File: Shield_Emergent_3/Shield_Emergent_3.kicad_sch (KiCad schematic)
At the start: 23 parts, among them J1 Conn_02x06_Counter_Clockwise

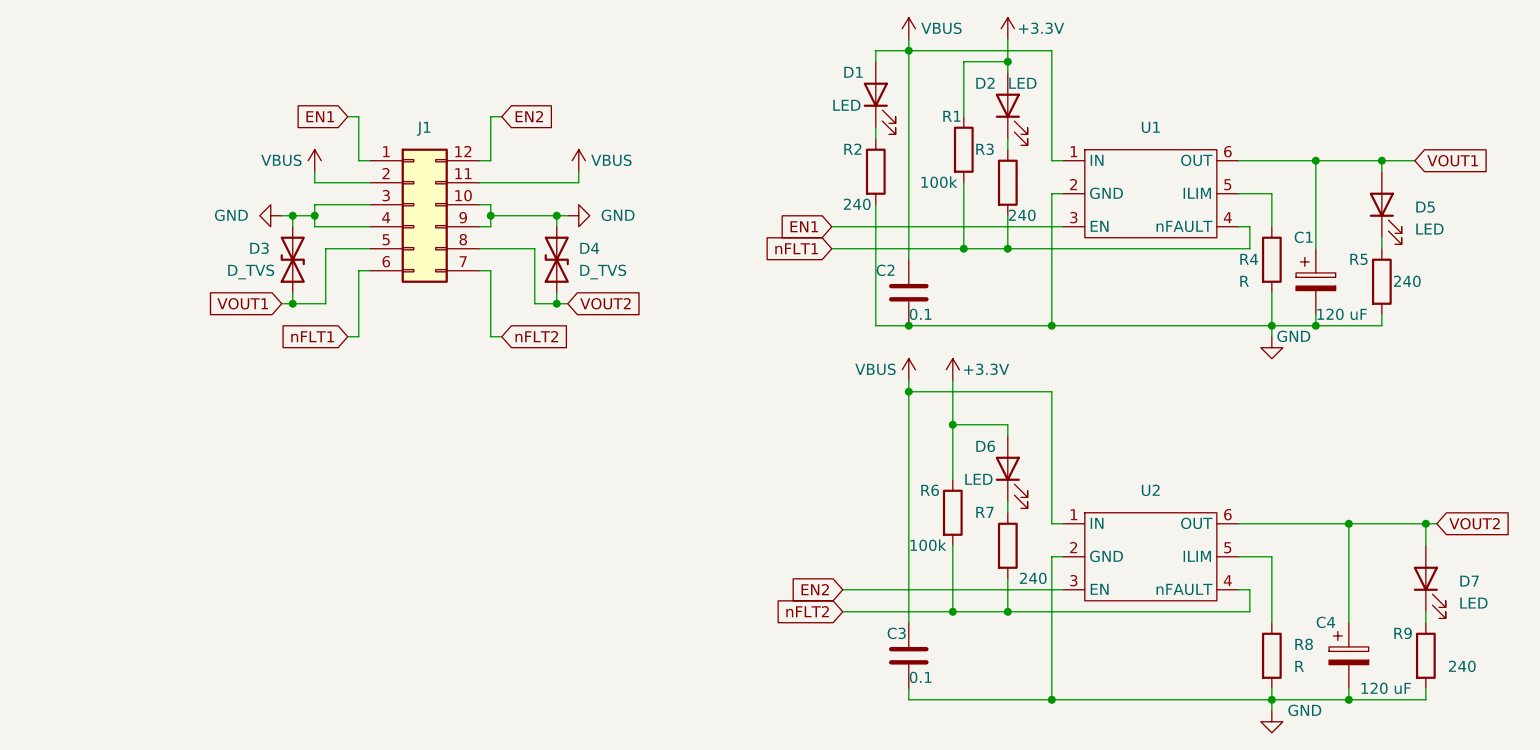
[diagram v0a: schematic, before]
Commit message: v0.2 some additions in the circuit
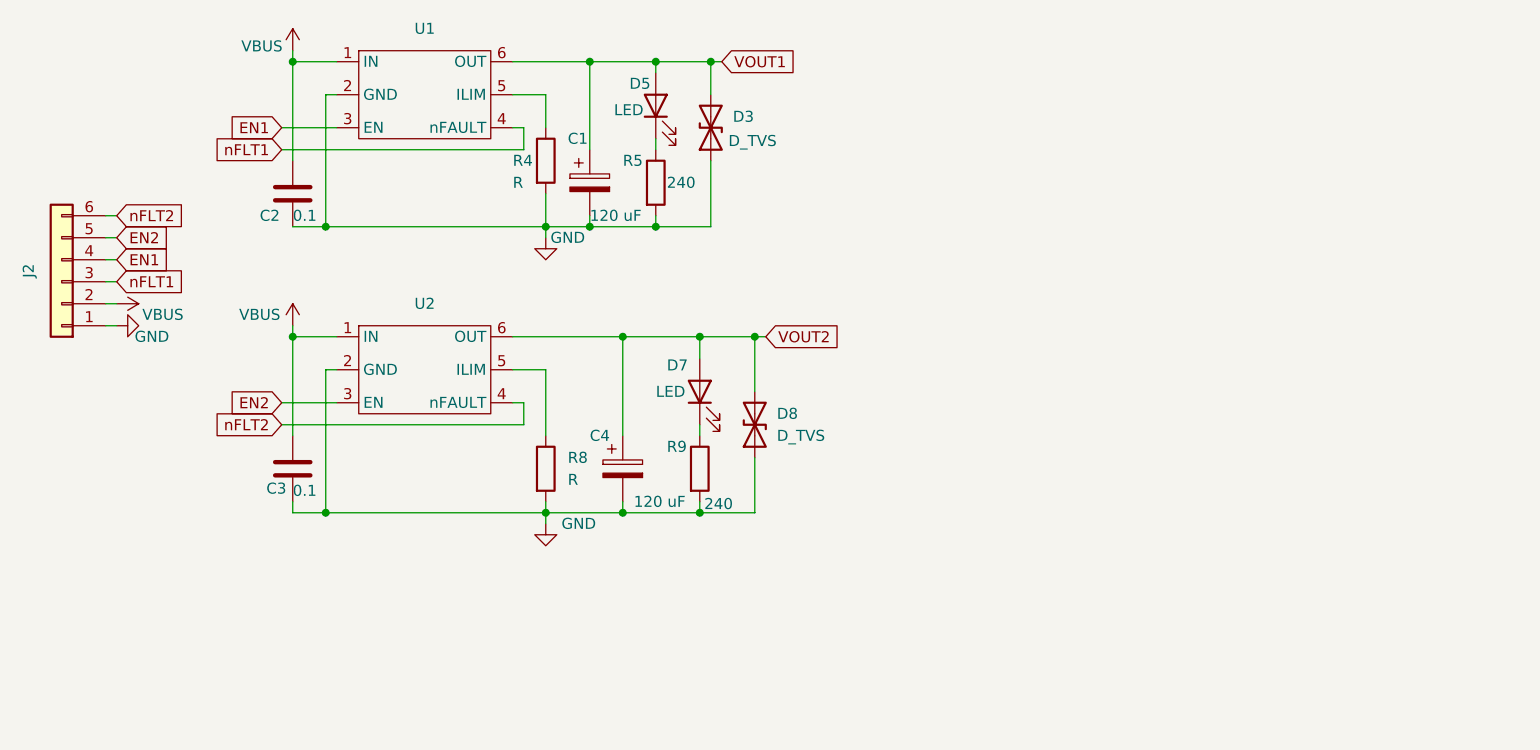
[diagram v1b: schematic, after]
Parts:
- removed D1, D2, D6: LED, LED_SMD:LED_0603_1608Metric_Pad1.05x0.95mm_HandSolder, symbol Device:LED
- removed D4: D_TVS, Diode_SMD:D_SOD-123F, symbol Device:D_TVS
- removed J1: Conn_02x06_Counter_Clockwise, symbol Connector_Generic:Conn_02x06_Counter_Clockwise
- removed R1, R6: 100k, Resistor_SMD:R_0603_1608Metric_Pad0.98x0.95mm_HandSolder, symbol Device:R
- removed R2, R3, R7: 240, Resistor_SMD:R_0603_1608Metric_Pad0.98x0.95mm_HandSolder, symbol Device:R
- added D8: D_TVS, Diode_SMD:D_SOD-123F, symbol Device:D_TVS
- added J2: Conn_01x06, Connector_PinHeader_2.54mm:PinHeader_1x06_P2.54mm_Vertical, symbol Connector_Generic:Conn_01x06
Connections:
- net EN1: now also J2.4 (Pin_4)
- net EN2: now also J2.5 (Pin_5)
- net GND: now also D3.1 (A1), D8.1 (A1), J2.1 (Pin_1); no longer D3.2 (A2)
- net VBUS: now also J2.2 (Pin_2)
- net VOUT1: now also D3.2 (A2); no longer D3.1 (A1)
- net VOUT2: now also D8.2 (A2)
- net nFLT1: now also J2.3 (Pin_3)
- net nFLT2: now also J2.6 (Pin_6)
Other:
- moved on the sheet: C1, C2, C3, C4, D5, D7, R4, R5, R8, R9, U1, U2
